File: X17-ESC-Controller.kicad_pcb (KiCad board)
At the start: 2 copper layers, 50 x 32 mm, 23 parts, among them IC1 STM32F091CCT7, J2 DF11-10DP-2DSA24, J3 DF11-10DP-2DSA24, J4 Conn_2Rows-05Pins, SW1 SW_Push, U1 8mHz, U2 MAX485CSA+T

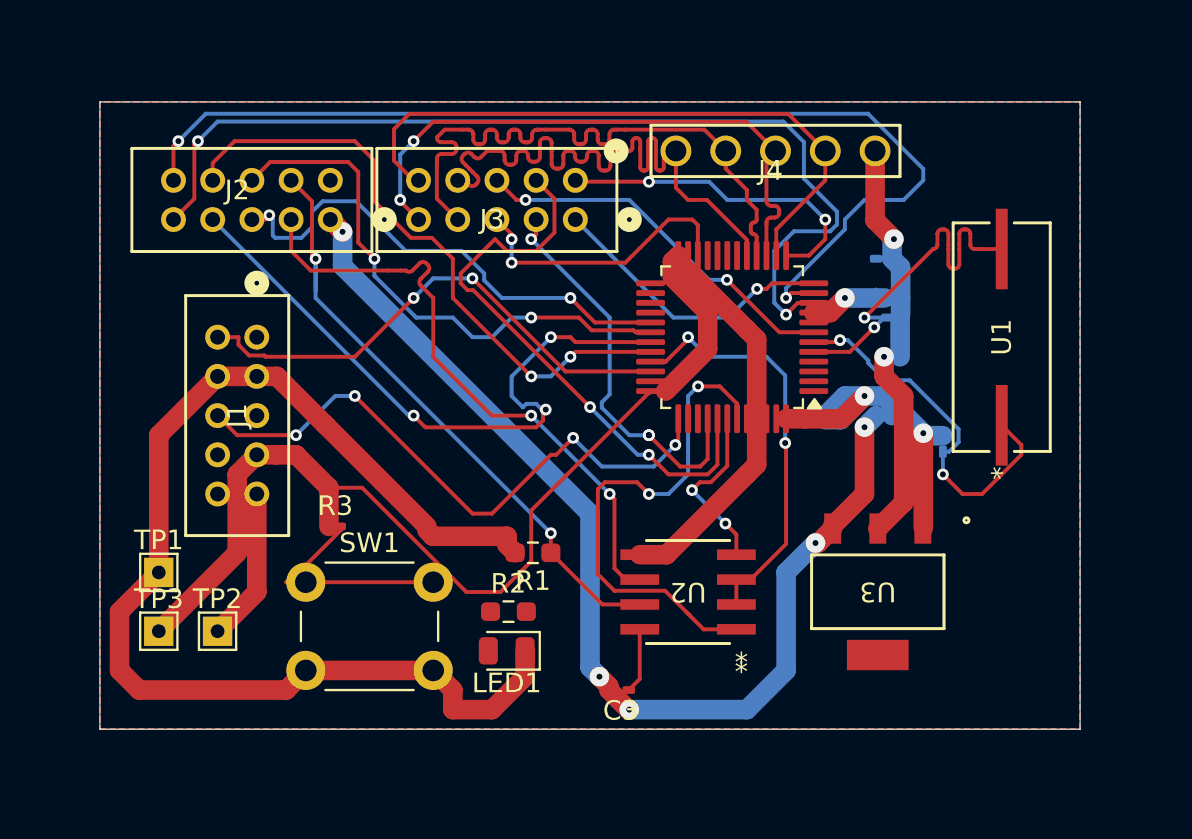
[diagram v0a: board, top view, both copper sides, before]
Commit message: layout fix
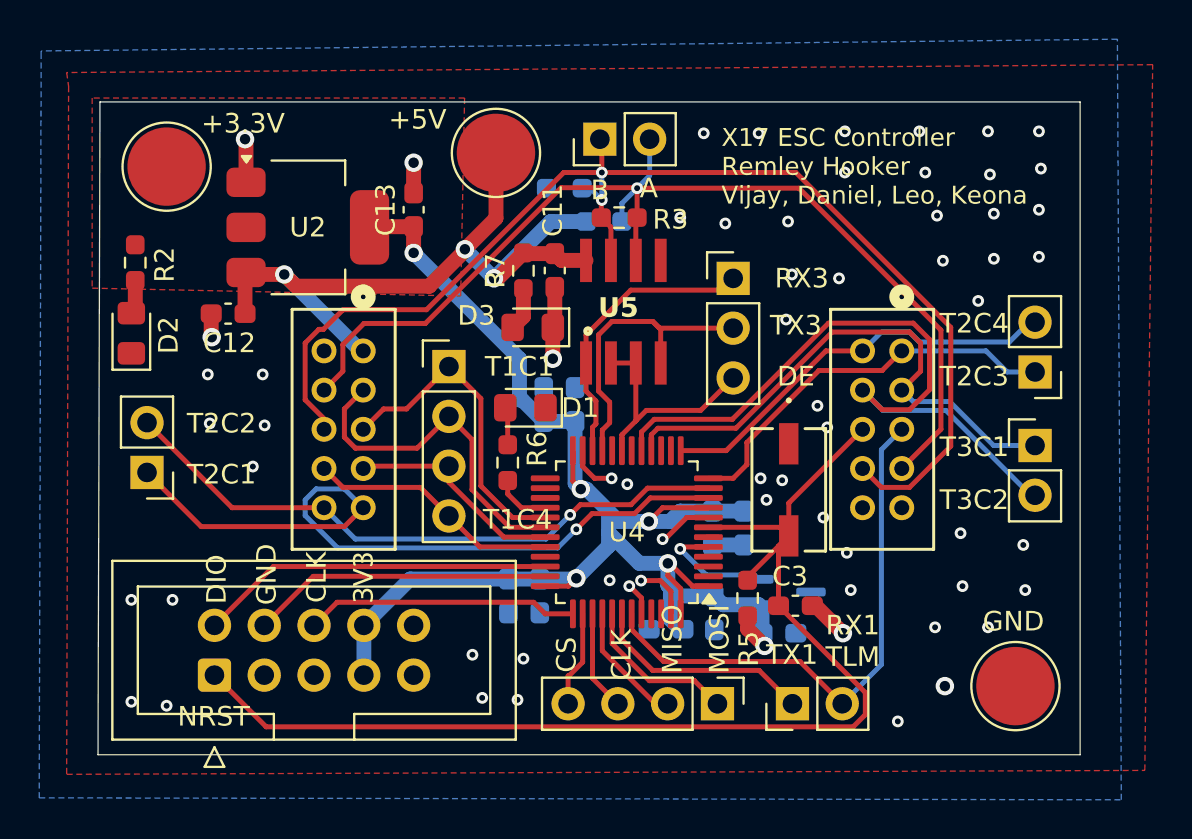
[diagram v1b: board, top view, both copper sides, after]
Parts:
- removed IC1: STM32F091CCT7, Package_QFP:LQFP-48_7x7mm_P0.5mm
- removed J2: DF11-10DP-2DSA24, Backplane:CON10_2X5_UF_DF11_HIR
- removed LED1: APT2012SGC, LED_SMD:LED_0805_2012Metric
- removed U1: 8mHz, Oscilator:ABLS-8.000MHZ-B2-T_ABR
- added C10: 4.7u, Capacitor_SMD:C_0603_1608Metric_Pad1.08x0.95mm_HandSolder, B.Cu at (149.2, 97.4)
- added C11: 0.1u, Capacitor_SMD:C_0603_1608Metric_Pad1.08x0.95mm_HandSolder, F.Cu at (148.2, 90.6)
- added C12: 10u, Capacitor_SMD:C_0603_1608Metric_Pad1.08x0.95mm_HandSolder, F.Cu at (131.5, 92.8)
- added C13: 22u, Capacitor_SMD:C_0603_1608Metric_Pad1.08x0.95mm_HandSolder, F.Cu at (141.0, 87.5)
- added C8: 0.1u, Capacitor_SMD:C_0603_1608Metric_Pad1.08x0.95mm_HandSolder, B.Cu at (153.9, 108.9)
- added C9: 4.7u, Capacitor_SMD:C_0603_1608Metric_Pad1.08x0.95mm_HandSolder, B.Cu at (145.8, 107.2)
- added D1: D, LED_SMD:LED_0805_2012Metric_Pad1.15x1.40mm_HandSolder, F.Cu at (146.7, 97.6)
- added D2: D, LED_SMD:LED_0805_2012Metric_Pad1.15x1.40mm_HandSolder, F.Cu at (126.6, 93.8)
- added D3: D, LED_SMD:LED_0805_2012Metric_Pad1.15x1.40mm_HandSolder, F.Cu at (147.1, 93.5)
- added J10: Conn_01x02, Connector_PinHeader_2.54mm:PinHeader_1x02_P2.54mm_Vertical, F.Cu at (127.4, 100.9)
- added J11: Conn_01x02, Connector_PinHeader_2.54mm:PinHeader_1x02_P2.54mm_Vertical, F.Cu at (172.7, 95.8)
- added J5: Conn_01x04, Connector_PinHeader_2.54mm:PinHeader_1x04_P2.54mm_Vertical, F.Cu at (156.5, 112.7)
- added J6: Conn_01x04, Connector_PinHeader_2.54mm:PinHeader_1x04_P2.54mm_Vertical, F.Cu at (142.8, 95.5)
- added J7: Conn_01x03, Connector_PinHeader_2.54mm:PinHeader_1x03_P2.54mm_Vertical, F.Cu at (157.3, 91.0)
- added J8: Conn_01x02, Connector_PinHeader_2.54mm:PinHeader_1x02_P2.54mm_Vertical, F.Cu at (150.5, 83.9)
- added J9: Conn_01x02, Connector_PinHeader_2.54mm:PinHeader_1x02_P2.54mm_Vertical, F.Cu at (160.3, 112.7)
- added R4: 10k, Resistor_SMD:R_0603_1608Metric_Pad0.98x0.95mm_HandSolder, B.Cu at (148.7, 86.4)
- added R5: 10k, Resistor_SMD:R_0603_1608Metric_Pad0.98x0.95mm_HandSolder, F.Cu at (158.0, 107.3)
- added R6: 100, Resistor_SMD:R_0603_1608Metric_Pad0.98x0.95mm_HandSolder, F.Cu at (145.8, 100.4)
- added R7: 240, Resistor_SMD:R_0603_1608Metric_Pad0.98x0.95mm_HandSolder, F.Cu at (146.6, 90.6)
- added U4: STM32F091CCTx, Package_QFP:LQFP-48_7x7mm_P0.5mm, F.Cu at (151.9, 104.0)
- added U5: MAX485, MAX485:SO08, F.Cu at (151.7, 92.7)
- C1: value 18pF -> 10n; footprint Capacitor_SMD:C_0201_0603Metric_Pad0.64x0.40mm_HandSolder -> Capacitor_SMD:C_0603_1608Metric_Pad1.08x0.95mm_HandSolder
- C2: value 18pF -> 0.1u; footprint Capacitor_SMD:C_0201_0603Metric_Pad0.64x0.40mm_HandSolder -> Capacitor_SMD:C_0603_1608Metric_Pad1.08x0.95mm_HandSolder
- C3: value CL10B104KB8NNWC -> 0.1u; footprint Capacitor_SMD:C_0201_0603Metric_Pad0.64x0.40mm_HandSolder -> Capacitor_SMD:C_0603_1608Metric_Pad1.08x0.95mm_HandSolder
- C4, C7: value C -> 0.1u; footprint Capacitor_SMD:C_0201_0603Metric_Pad0.64x0.40mm_HandSolder -> Capacitor_SMD:C_0603_1608Metric_Pad1.08x0.95mm_HandSolder
- C5: value GRM188R60G226MEA0D -> 0.1u; footprint Capacitor_SMD:C_0201_0603Metric_Pad0.64x0.40mm_HandSolder -> Capacitor_SMD:C_0603_1608Metric_Pad1.08x0.95mm_HandSolder
- C6: value GRM188R60G226MEA0D -> 1u; footprint Capacitor_SMD:C_0201_0603Metric_Pad0.64x0.40mm_HandSolder -> Capacitor_SMD:C_0603_1608Metric_Pad1.08x0.95mm_HandSolder
- J1: footprint ST Link:CON10_2X5_UF_DF11_HIR -> Backplane Connector:CON10_2X5_UF_DF11_HIR
- J3: value DF11-10DP-2DSA24 -> Conn_01x02; footprint Backplane:CON10_2X5_UF_DF11_HIR -> Connector_PinHeader_2.54mm:PinHeader_1x02_P2.54mm_Vertical
- J4: value Conn_2Rows-05Pins -> Conn_02x05_Odd_Even; footprint footprints:CONN_A-4030-05A_MOL -> Connector_IDC:IDC-Header_2x05_P2.54mm_Vertical
- R1: value 20k -> 10k; moved to B.Cu
- R2: value 4.2k -> 100
- R3: value 10k -> 120; footprint Resistor_SMD:R_0201_0603Metric -> Resistor_SMD:R_0603_1608Metric_Pad0.98x0.95mm_HandSolder
- SW1: footprint Button_Switch_THT:SW_PUSH_6mm -> Button-SW_FSM2JMTR_TEC:SW_FSM2JMTR_TEC
- TP1, TP2, TP3: footprint TestPoint:TestPoint_THTPad_1.5x1.5mm_Drill0.7mm -> TestPoint:TestPoint_Pad_D4.0mm
- U2: value MAX485CSA+T -> AZ1117-3.3; footprint MAX45:21-0041-3-M_90-0096-8L_MXM -> Package_TO_SOT_SMD:SOT-223-3_TabPin2
- U3: value ~ -> MAX7375AXR805; footprint A1117IH:SOT223_AZ1117I_6P5X3P5_DIO -> Package_TO_SOT_SMD:SOT-323_SC-70_Handsoldering; moved to B.Cu
- moved TP1 44.1 mm to (171.7, 111.8)
- moved J4 35.6 mm to (130.8, 111.2), turned to 90 degrees
- moved TP2 28.2 mm to (145.2, 84.6)
- moved U2 26.9 mm to (135.6, 88.4), turned to 0 degrees
- moved J3 26.1 mm to (172.7, 99.5)
- moved R2 26.1 mm to (126.8, 90.2), turned to 90 degrees
- moved SW1 25.1 mm to (160.1, 101.8), turned to -90 degrees
- moved C4 24.6 mm to (147.4, 107.2), turned to -90 degrees
- moved TP3 23.7 mm to (128.4, 85.3)
- moved R3 21.4 mm to (151.5, 87.9)
- moved C2 18.5 mm to (147.6, 97.4), turned to 90 degrees
- moved C7 18.5 mm to (156.3, 108.1), turned to -90 degrees
- moved R1 17.3 mm to (150.7, 88.1)
- moved C6 12.7 mm to (156.2, 103.7), turned to -90 degrees
- moved C5 12.3 mm to (159.6, 109.1), turned to 0 degrees
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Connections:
- C1 pad 1: RCC_OSC_OUT -> +3.3V
- C2 pad 1: RCC_OSC_IN -> +3.3V
- C3 pad 1: Net-(U2-VCC) -> NRST
- C3 pad 2: +5V -> GND
- C4 pad 1: GND -> +3.3V
- C4 pad 2: +3.3V -> GND
- C5 pad 1: GND -> +3.3V
- C5 pad 2: +5V -> GND
- C6 pad 1: /-3.3V -> +3.3V
- C7 pad 1: GND -> +3.3V
- C7 pad 2: +3.3V -> GND
- J1 pad 1: /NC -> +5V
- J1 pad 10: /NC -> TIM2_CH2
- J1 pad 2: SYS_SWDIO -> GND
- J1 pad 3: GND -> TIM1_CH2
- J1 pad 4: GND -> A
- J1 pad 5: /NC -> TIM1_CH1
- J1 pad 6: SWCLK -> B
- J1 pad 7: +3.3V -> TIM1_CH3
- J1 pad 8: /NC -> TIM1_CH4
- J1 pad 9: +5.0V -> TIM2_CH1
- J3 pad 1: TIM2_CH3 -> TIM3_CH1
- J3 pad 2: TIM2_CH4 -> TIM3_CH2
- J4 pad 1: MOSI -> NRST
- J4 pad 2: MISO -> SYS_SWDIO
- J4 pad 3: SCLK -> GND
- J4 pad 4: CS -> GND
- J4 pad 5: GND -> unconnected-(J4-Pin_5-Pad5)
- R1 pad 1: B -> A
- R1 pad 2: GND -> +5V
- R2 pad 1: LED -> Net-(D2-A)
- R2 pad 2: Net-(LED1-Pad2) -> +3.3V
- R3 pad 1: +3.3V -> B
- R3 pad 2: NRST -> A
- SW1 pad 1: NRST -> GND
- SW1 pad 2: GND -> NRST
- TP2 pad 1: +5.0V -> +5V
- U2 pad 1: USART1_RX -> GND
- U2 pad 2: USART1_DE -> +3.3V
- U2 pad 3: USART1_DE -> +5V
- U3 pad 1: GND -> +3.3V
- U3 pad 2: /-3.3V -> RCC_OSC_IN
- U3 pad 3: +5V -> GND
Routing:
- net GND: track 93.0 -> 37.7 mm, vias 1 -> 63
- net +5V: track 74.9 -> 40.2 mm, vias 7 -> 3
- net B: track 31.7 -> 64.3 mm
- net NRST: track 30.0 -> 60.1 mm, vias 2 -> 0
- net CS: track 32.8 -> 4.92 mm
- net MISO: track 32.7 -> 6.34 mm
- net MOSI: track 33.8 -> 8.16 mm
- net SCLK: track 30.6 -> 5.12 mm, vias 2 -> 0
- net A: track 31.7 -> 55.9 mm, vias 2 -> 1
- net +3.3V: track 53.2 -> 77.2 mm, vias 1 -> 6
- net TIM1_CH3: track 33.3 -> 11.3 mm, vias 3 -> 0
- net TIM2_CH2: track 54.0 -> 32.2 mm, vias 2 -> 1
- net USART1_DE: track 21.4 -> 0.00 mm, vias 2 -> 0
- net RCC_OSC_OUT: track 19.4 -> 0.00 mm, vias 2 -> 0
- net TIM1_CH4: track 31.6 -> 12.9 mm, vias 2 -> 0
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- removed copper zone on B.Cu, net +5.0V
- removed copper zone on F.Cu, net +5.0V
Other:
- board size 50 x 32 mm -> 50.1 x 33.3 mm
- board text added: "+3.3V"
- board text added: "+5V"
- board text added: "3V3"
- board text added: "A"
- board text added: "B"
- board text added: "CLK"
- board text added: "CS"
- board text added: "DE"
- board text added: "DIO"
- board text added: "GND"
- board text added: "MISO"
- board text added: "MOSI"
- board text added: "NRST"
- board text added: "RX1 TLM"
- board text added: "RX3"
- board text added: "T1C1"
- board text added: "T1C4"
- board text added: "T2C1"
- board text added: "T2C2"
- board text added: "T2C3"
- board text added: "T2C4"
- board text added: "T3C1"
- board text added: "T3C2"
- board text added: "TX1"
- board text added: "TX3"
- board text added: "X17 ESC Controller Remley Hooker Vijay, Daniel, Leo, Keona"
